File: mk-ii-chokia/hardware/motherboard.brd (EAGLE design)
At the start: 100 x 80 mm, 10 parts, among them T2 BC337

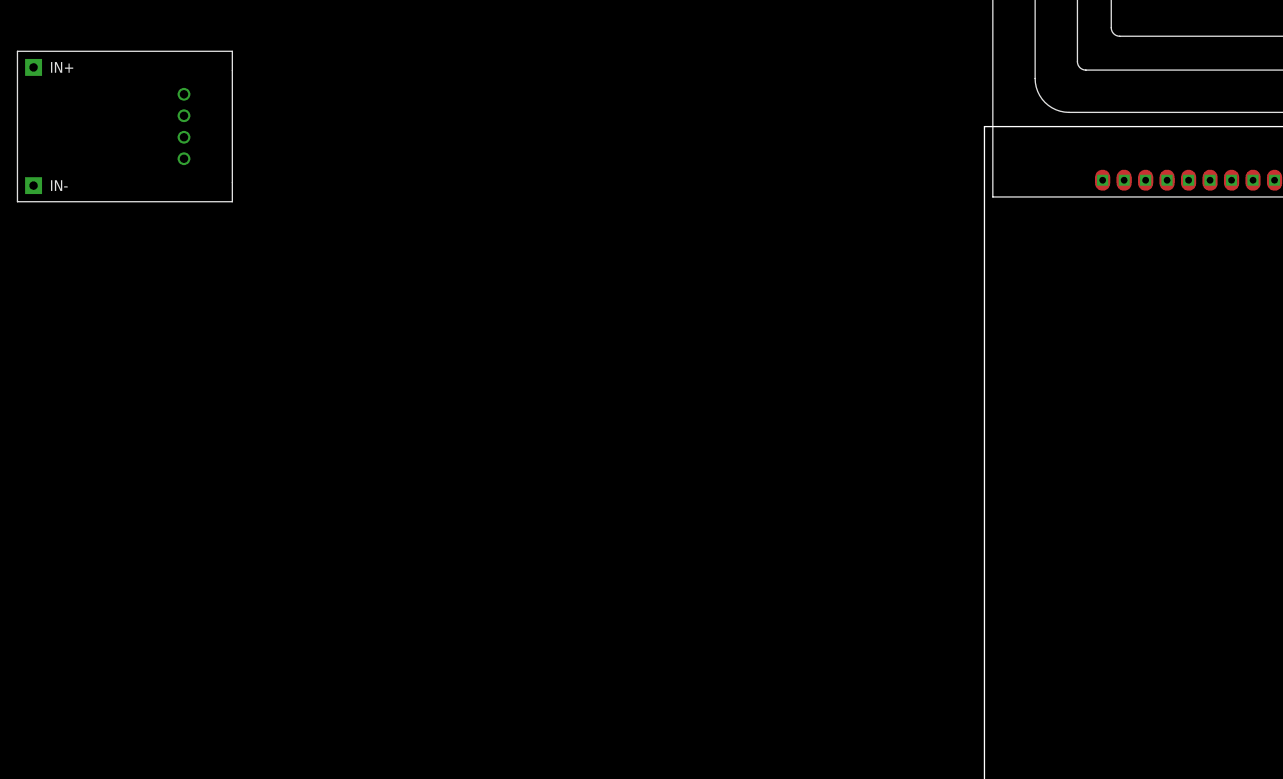
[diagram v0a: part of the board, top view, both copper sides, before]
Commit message: Chokia sends. Pager receives. Not vice-versa...
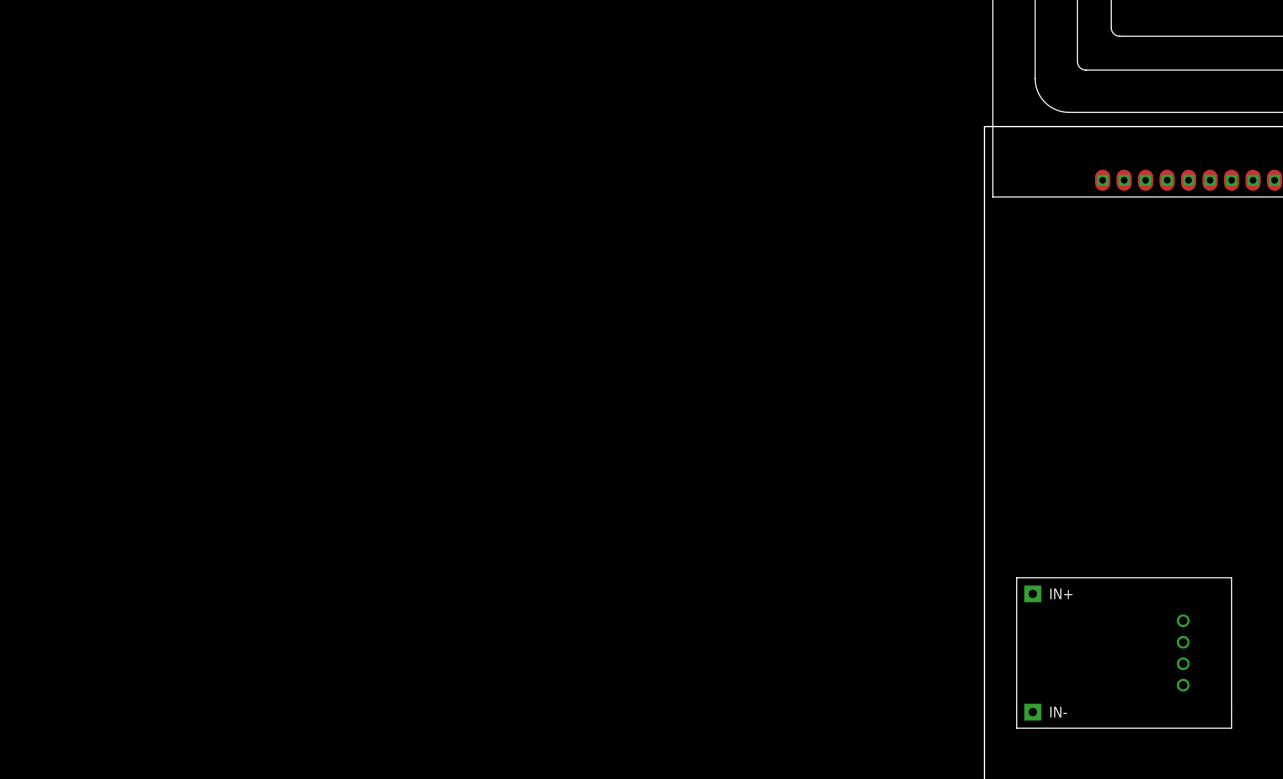
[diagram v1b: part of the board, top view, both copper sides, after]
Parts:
- moved U$5 133.5 mm to (16.5, 17.8)
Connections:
- removed net N$31: T2.1, U$1.19
- new net N$14: T2.3, U$1.20
- new net N$17: U$2.P$7
- net +5V: now also U$1.19
- net GND: now also T2.1; no longer U$1.20
- net N$15: now also U$2.P$6; no longer T2.3
- net N$18: now also U$2.P$36; no longer U$2.P$37
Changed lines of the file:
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@@
 </element>
 <element name="U$4" library="lora-ra-02-minimal-because-labels-fuckup-rotating" package="AI-THINKER_RA-01" value="AI-THINKER_RA-01" x="-22.86" y="132.08" smashed="yes"/>
-<element name="U$5" library="5v-step-up-minimal" package="DC-DC-STEP-UP-5V" value="DC-DC-STEP-UP-5V" x="-101.6" y="80.01" smashed="yes"/>
+<element name="U$5" library="5v-step-up-minimal" package="DC-DC-STEP-UP-5V" value="DC-DC-STEP-UP-5V" x="16.51" y="17.78" smashed="yes"/>
 <element name="T2" library="transistor" library_urn="urn:adsk.eagle:library:402" package="TO92" package3d_urn="urn:adsk.eagle:package:28523/2" value="BC337" x="-110.49" y="-10.16" smashed="yes">
 <attribute name="NAME" x="-107.315" y="-9.525" size="1.27" layer="25" ratio="10"/>
@@
 <contactref element="U$2" pad="P$22"/>
 <contactref element="U$1" pad="1"/>
-<contactref element="U$1" pad="20"/>
+<contactref element="T2" pad="1"/>
 <wire x1="58.42" y1="49.53" x2="62.23" y2="73.66" width="0" layer="19" extent="1-1"/>
 <wire x1="92.075" y1="26.035" x2="58.42" y2="49.53" width="0" layer="19" extent="1-1"/>
 <wire x1="43.18" y1="6.35" x2="58.42" y2="49.53" width="0" layer="19" extent="1-1"/>
-<wire x1="13.97" y1="73.66" x2="62.23" y2="73.66" width="0" layer="19" extent="1-1"/>
-<wire x1="-14.86" y1="139.08" x2="13.97" y2="73.66" width="0" layer="19" extent="1-1"/>
+<wire x1="-14.86" y1="139.08" x2="62.23" y2="73.66" width="0" layer="19" extent="1-1"/>
 <wire x1="-13.96" y1="143.51" x2="-14.86" y2="139.08" width="0" layer="19" extent="1-1"/>
 <wire x1="-30.86" y1="137.08" x2="-14.86" y2="139.08" width="0" layer="19" extent="1-1"/>
-<wire x1="-94.615" y1="83.82" x2="-30.86" y2="137.08" width="0" layer="19" extent="1-1"/>
-<wire x1="-112.395" y1="73.025" x2="-94.615" y2="83.82" width="0" layer="19" extent="1-1"/>
+<wire x1="23.495" y1="21.59" x2="-30.86" y2="137.08" width="0" layer="19" extent="1-1"/>
+<wire x1="5.715" y1="10.795" x2="23.495" y2="21.59" width="0" layer="19" extent="1-1"/>
+<wire x1="-109.22" y1="-10.16" x2="5.715" y2="10.795" width="0" layer="19" extent="1-1"/>
 </signal>
 <signal name="+5V">
@@
 <contactref element="U$2" pad="P$18"/>
 <contactref element="U$1" pad="2"/>
-<wire x1="-94.615" y1="76.2" x2="58.42" y2="46.99" width="0" layer="19" extent="1-1"/>
-<wire x1="59.69" y1="73.66" x2="58.42" y2="46.99" width="0" layer="19" extent="1-1"/>
+<contactref element="U$1" pad="19"/>
+<wire x1="58.42" y1="46.99" x2="59.69" y2="73.66" width="0" layer="19" extent="1-1"/>
+<wire x1="16.51" y1="73.66" x2="59.69" y2="73.66" width="0" layer="19" extent="1-1"/>
+<wire x1="23.495" y1="13.97" x2="16.51" y2="73.66" width="0" layer="19" extent="1-1"/>
 </signal>
 <signal name="N$16">
@@
 <contactref element="U$5" pad="IN+"/>
 <wire x1="-100.34" y1="125.73" x2="-34.29" y2="125.73" width="0" layer="19" extent="1-1"/>
-<wire x1="-112.395" y1="86.995" x2="-100.34" y2="125.73" width="0" layer="19" extent="1-1"/>
+<wire x1="5.715" y1="24.765" x2="-100.34" y2="125.73" width="0" layer="19" extent="1-1"/>
 </signal>
 <signal name="N$1">
@@
 <wire x1="-107.95" y1="-3.81" x2="-110.49" y2="-8.255" width="0" layer="19" extent="1-1"/>
 </signal>
+<signal name="N$18">
+<contactref element="U$2" pad="P$36"/>
+<contactref element="R1" pad="1"/>
+<wire x1="43.18" y1="41.91" x2="-113.03" y2="-3.81" width="0" layer="19" extent="1-1"/>
+</signal>
+<signal name="N$14">
+<contactref element="U$1" pad="20"/>
+<contactref element="T2" pad="3"/>
+<wire x1="13.97" y1="73.66" x2="-111.76" y2="-10.16" width="0" layer="19" extent="1-1"/>
+</signal>
 <signal name="N$15">
-<contactref element="T2" pad="3"/>
+<contactref element="U$2" pad="P$6"/>
 </signal>
-<signal name="N$18">
-<contactref element="U$2" pad="P$37"/>
-<contactref element="R1" pad="1"/>
-<wire x1="43.18" y1="44.45" x2="-113.03" y2="-3.81" width="0" layer="19" extent="1-1"/>
-</signal>
-<signal name="N$31">
-<contactref element="T2" pad="1"/>
-<contactref element="U$1" pad="19"/>
-<wire x1="16.51" y1="73.66" x2="-109.22" y2="-10.16" width="0" layer="19" extent="1-1"/>
+<signal name="N$17">
+<contactref element="U$2" pad="P$7"/>
 </signal>
 </signals>
